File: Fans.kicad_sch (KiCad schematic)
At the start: 18 parts, among them Q1 BUK7M27-80EX, Q2 BUK7M27-80EX, U2 EMC2305-1-AP-TR

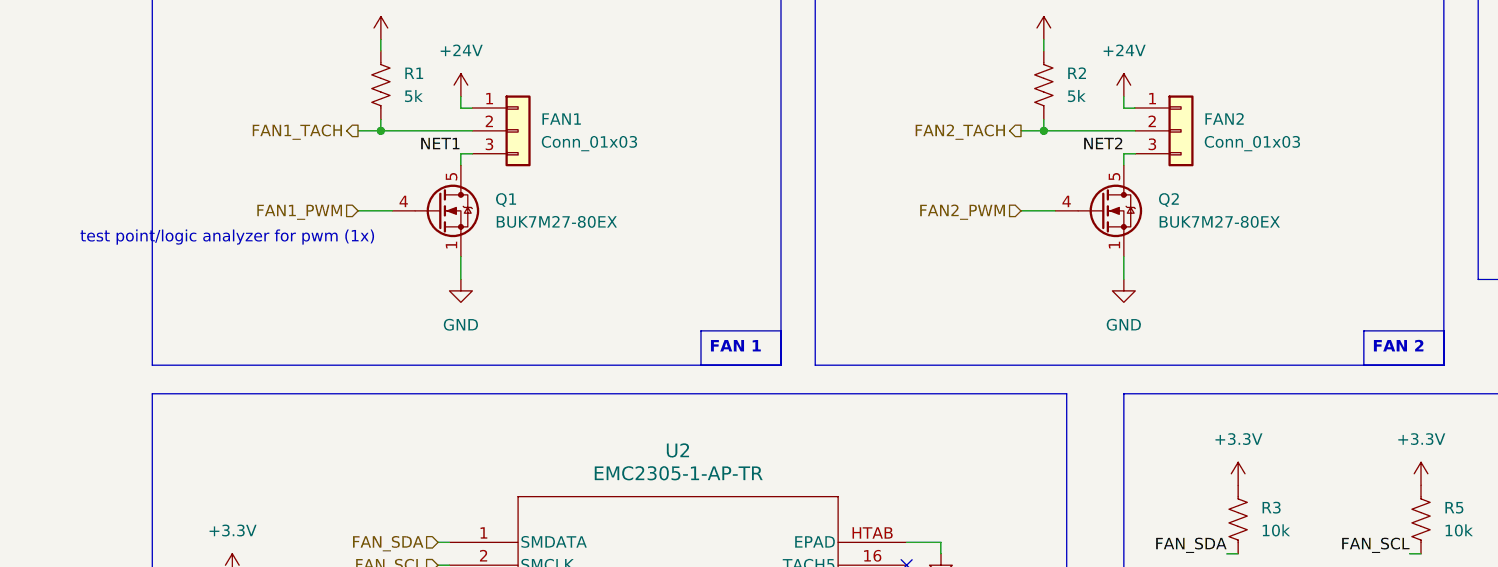
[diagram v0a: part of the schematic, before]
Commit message: schematic changes before switching submodules
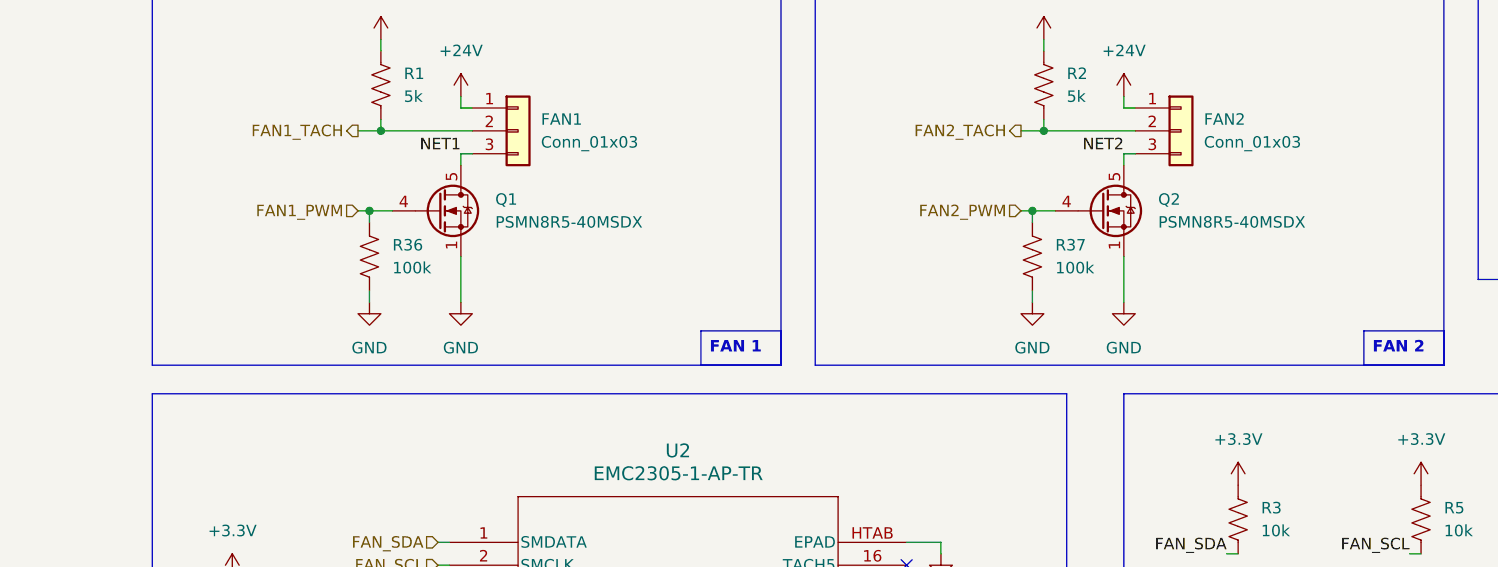
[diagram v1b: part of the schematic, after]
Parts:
- added R36, R37: 100k, Resistor_SMD:R_0603_1608Metric, symbol Device:R_US
- Q1, Q2: value BUK7M27-80EX -> PSMN8R5-40MSDX
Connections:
- net FAN1_PWM: now also R36.1
- net FAN2_PWM: now also R37.1
- net GND: now also R36.2, R37.2
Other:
- note removed: "test point/logic analyzer for pwm (1x)"

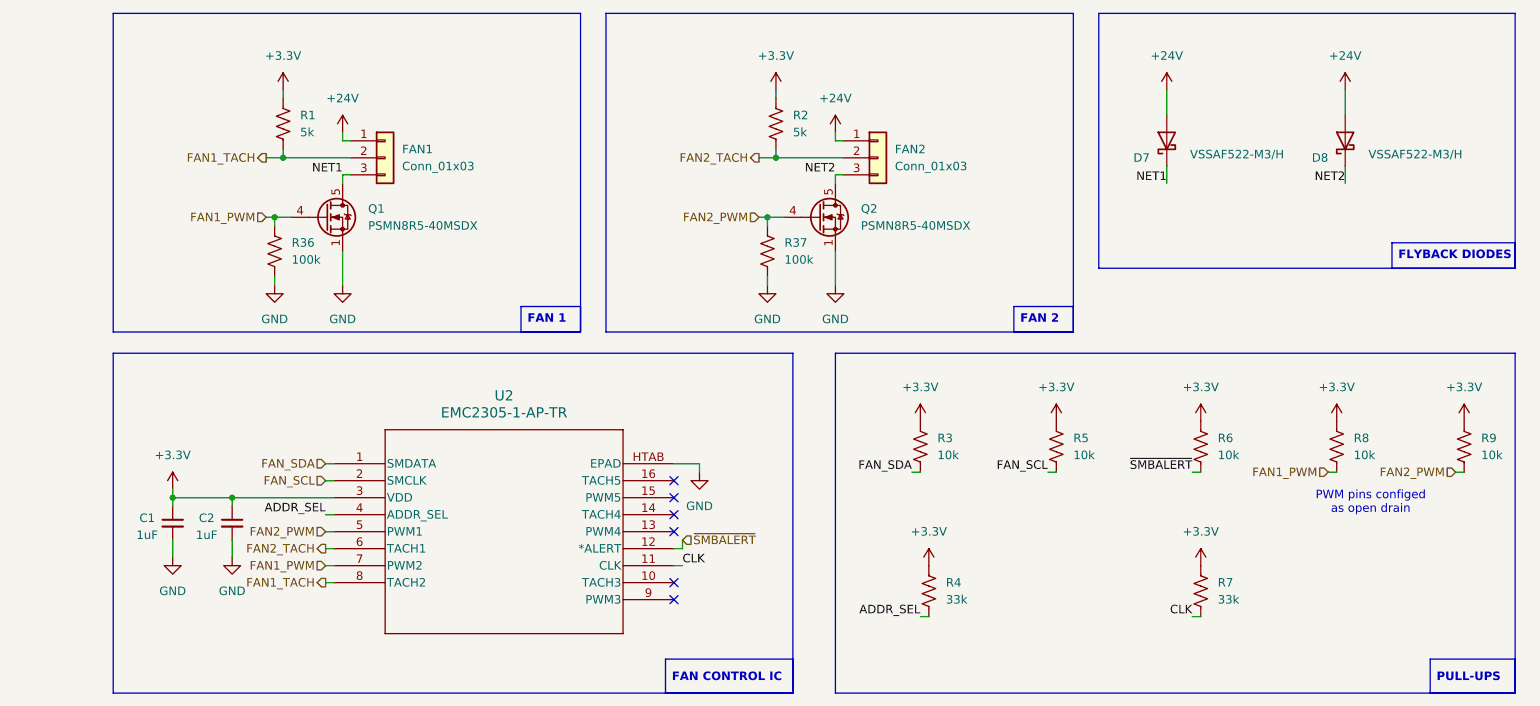
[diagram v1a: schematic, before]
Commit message: fixed submodule, schematic basically done
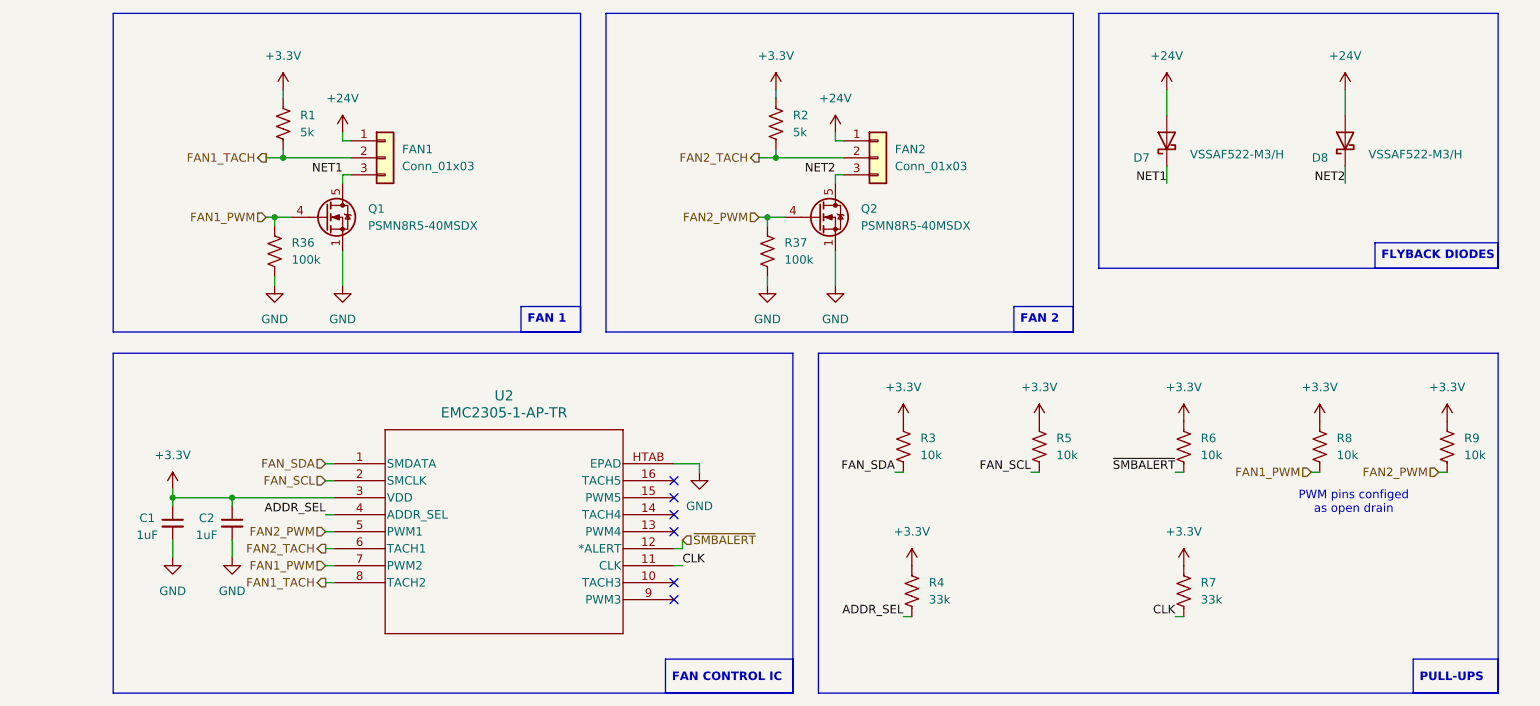
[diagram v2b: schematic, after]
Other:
- moved on the sheet: R3, R4, R5, R6, R7, R8, R9
